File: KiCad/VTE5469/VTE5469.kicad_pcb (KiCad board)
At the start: 2 copper layers, 72.5 x 53.8 mm, 34 parts, among them J1 Power, J2 JRD-100 (UHF RFID), J3 Program, J4 Display, Q1 BD138, Q3 BC547, SW1 Switch, SW2 Reset, SW3 Mode, U1 AMS1117-3.3, U2 ESP-12F, U3 MQ-2, U4 Vibration, U5 XD-58C, U6 DHT11

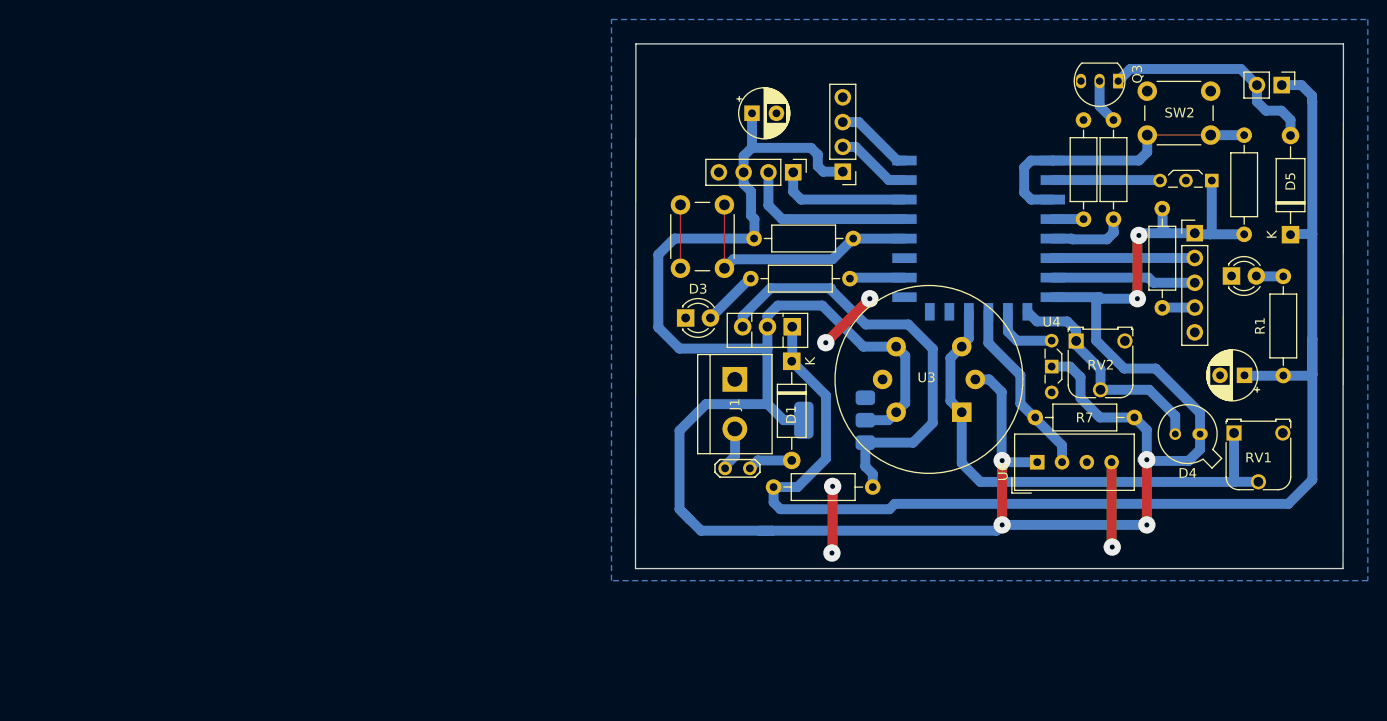
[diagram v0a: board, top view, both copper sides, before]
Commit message: Updates
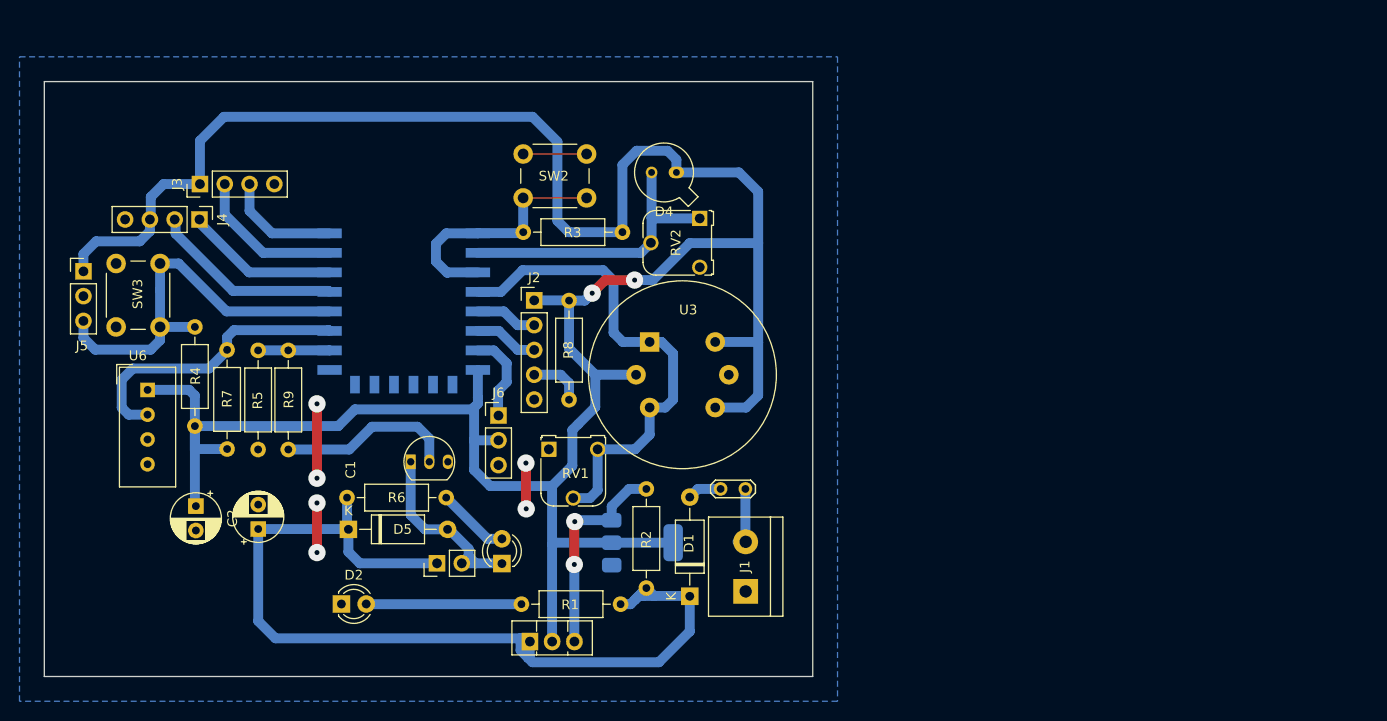
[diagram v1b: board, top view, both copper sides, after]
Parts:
- removed U4: Vibration, Sensor_Current:Diodes_SIP-3_4.1x1.5mm_P2.65mm
- removed U5: XD-58C, Sensor_Current:Diodes_SIP-3_4.1x1.5mm_P2.65mm
- added J5: Vibration, Connector_PinHeader_2.54mm:PinHeader_1x03_P2.54mm_Vertical, F.Cu at (123.4, 105.8)
- added J6: XD-58C, Connector_PinHeader_2.54mm:PinHeader_1x03_P2.54mm_Vertical, F.Cu at (165.9, 120.6)
- moved C1 102.3 mm to (141.3, 132.2), turned to 90 degrees
- moved D5 101.2 mm to (150.5, 132.2), turned to 0 degrees
- moved BZ2 99.5 mm to (159.6, 135.7), turned to 90 degrees
- moved D2 97.2 mm to (149.8, 139.9)
- moved R7 93.0 mm to (138.1, 124.0), turned to 90 degrees
- moved U6 91.5 mm to (130.0, 118.0), turned to 0 degrees
- moved R5 85.6 mm to (141.3, 113.9), turned to -90 degrees
- moved R9 85.6 mm to (144.4, 113.9), turned to -90 degrees
- moved Q3 81.2 mm to (157.6, 125.3), turned to 0 degrees
- moved R1 71.8 mm to (178.4, 139.9), turned to 180 degrees
- moved RV1 70.2 mm to (171.1, 124.0)
- moved C2 69.8 mm to (134.9, 129.9), turned to -90 degrees
- moved J2 68.0 mm to (169.6, 108.8)
- moved J3 65.9 mm to (135.3, 96.9), turned to 90 degrees
- moved SW2 64.3 mm to (168.4, 93.8)
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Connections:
- D3 pad 1: GND -> Net-(BZ2--)
- R4 pad 2: Net-(SW3-A) -> /vibr_pin
- R5 pad 1: Net-(U2-GPIO16) -> Net-(U2-GPIO15)
- R6 pad 1: Net-(U2-GPIO15) -> +7.4V
- R9 pad 1: Net-(U2-GPIO14) -> Net-(U2-GPIO15)
- RV1 pad 1: Net-(U2-GPIO10) -> GND
- RV1 pad 2: Net-(U2-GPIO10) -> /mq2
- RV1 pad 3: GND -> /mq2
- SW3 pad 1: Net-(SW3-A) -> /vibr_pin
- U2 pad 10: /vibr_pin -> unconnected-(U2-MISO-Pad10)
- U2 pad 11: /temp_pin -> unconnected-(U2-GPIO9-Pad11)
- U2 pad 12: Net-(U2-GPIO10) -> unconnected-(U2-GPIO10-Pad12)
- U2 pad 17: unconnected-(U2-GPIO2-Pad17) -> /temp_pin
- U2 pad 18: Net-(SW3-A) -> /vibr_pin
- U2 pad 2: /hb_pin -> /frame_pin
- U2 pad 4: Net-(U2-GPIO16) -> /mq2
- U2 pad 5: Net-(U2-GPIO14) -> /rfid_tx
- U2 pad 6: /rfid_tx -> /rfid_rx
- U2 pad 7: /rfid_rx -> /hb_pin
- U2 pad 9: /frame_pin -> unconnected-(U2-CS0-Pad9)
- U3 pad 1: Net-(U2-GPIO10) -> /mq2
- U3 pad 3: Net-(U2-GPIO10) -> /mq2
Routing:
- net Net-(U2-GPIO10): track 53.5 -> 0.00 mm
- net /mq2: track 0.00 -> 50.8 mm
- net +7.4V: track 135.8 -> 99.1 mm
- net /vibr_pin: track 6.91 -> 41.3 mm
- net Net-(SW3-A): track 26.2 -> 0.00 mm
- net Net-(Q1-B): track 44.6 -> 21.5 mm, vias 0 -> 2
- net Net-(Q3-B): track 4.58 -> 18.3 mm
- net Net-(D2-A): track 2.78 -> 15.9 mm
- net +3.3V: track 271.5 -> 284.3 mm, vias 6 -> 2
- net /temp_pin: track 18.5 -> 30.0 mm
- net /rfid_tx: track 14.6 -> 6.35 mm
- net /rfid_rx: track 14.8 -> 6.58 mm
- net Net-(U2-GPIO14): track 7.96 -> 0.00 mm
- net /Rx: track 7.73 -> 15.5 mm
- net /frame_pin: track 23.5 -> 30.3 mm
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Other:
- board size 72.5 x 53.8 mm -> 78.7 x 61 mm
